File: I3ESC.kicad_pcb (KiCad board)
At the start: 4 copper layers, 82 x 54 mm, 185 parts, among them J1 JST SR/SZ, J10 VIN_BARREL, J11 Barrel_Jack, J12 JST SR/SZ, J13 Conn_01x04, J2 Screw_Terminal_01x02, J3 Screw_Terminal_01x02, J4 Screw_Terminal_01x02, J5 Conn_01x06, J6 Wireless Coil, J7 VIN_TERMINAL, J8 Conn_01x06, J9 JST SR/SZ, SW2 boot-red, SW3 user1-white, U1 SY8113BADC, U10 USBLC6-2P6, U11 IP6826, U12 FD8288T (DRV8300), U2 FD8288T (DRV8300), U3 SPX3819M5-L-3-3, U4 STM32G474RETx, U5 Qwiic1, U6 USB_C_Receptacle, U8 ABM3B-8.000MHZ, U9 USB_C_Receptacle

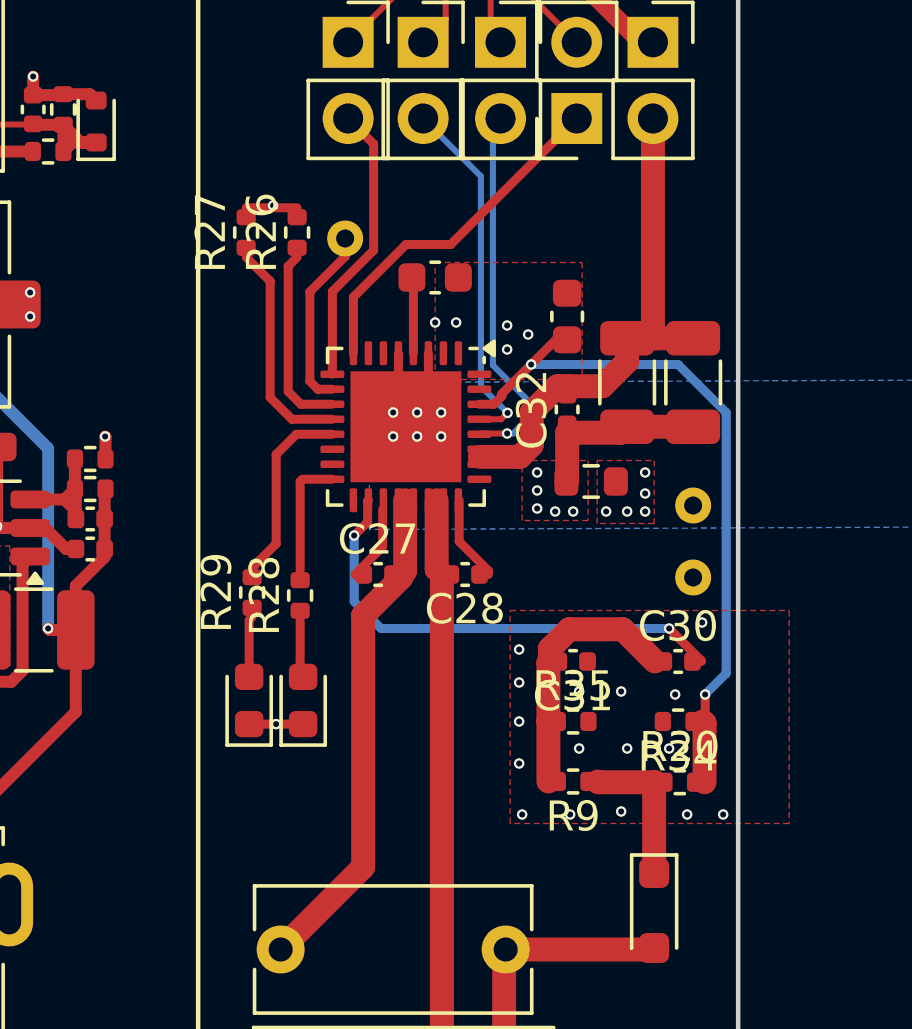
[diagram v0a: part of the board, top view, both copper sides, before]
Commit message: cleaned up all files, created schematic PDF
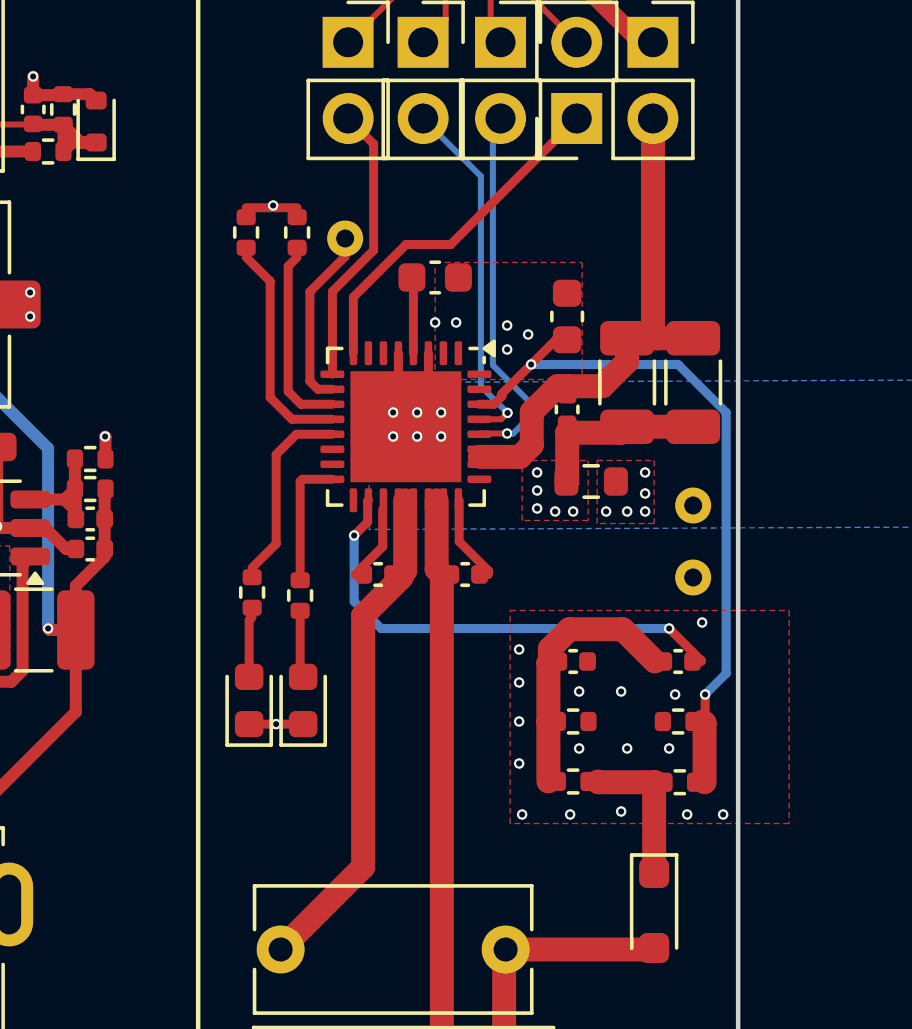
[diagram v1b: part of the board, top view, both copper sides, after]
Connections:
- net /PGND renamed /IE-QI-WIRELESS/PGND
- net /V_QI_USB renamed /IE-QI-WIRELESS/V_QI_USB
